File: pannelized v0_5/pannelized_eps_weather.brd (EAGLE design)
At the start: 95.5 x 64 mm, 169 parts, among them IC1 OPA2333DGK, IC100 OPA2333DGK, IC101 OPA347, IC2 OPA2333DGK, Q1 N-HEXFET-2D_SOT232-, Q100 N-HEXFET-2D_SOT232-, Q2 N-HEXFET-2D_SOT232-, Q3 FC-12M, Q4 32.768kHz, Q5 32.768kHz, U1 BMP180, U10 ML8511-UV-SENSORSMD, U11 AS3935, U12 BNO055A, U2 SHT21, U3 ML8511-UV-SENSORSMD, U4 MCP3425, U5 BNO055A, U6 AS3935, U7 SHT21, U8 BMP180, U9 MCP3425

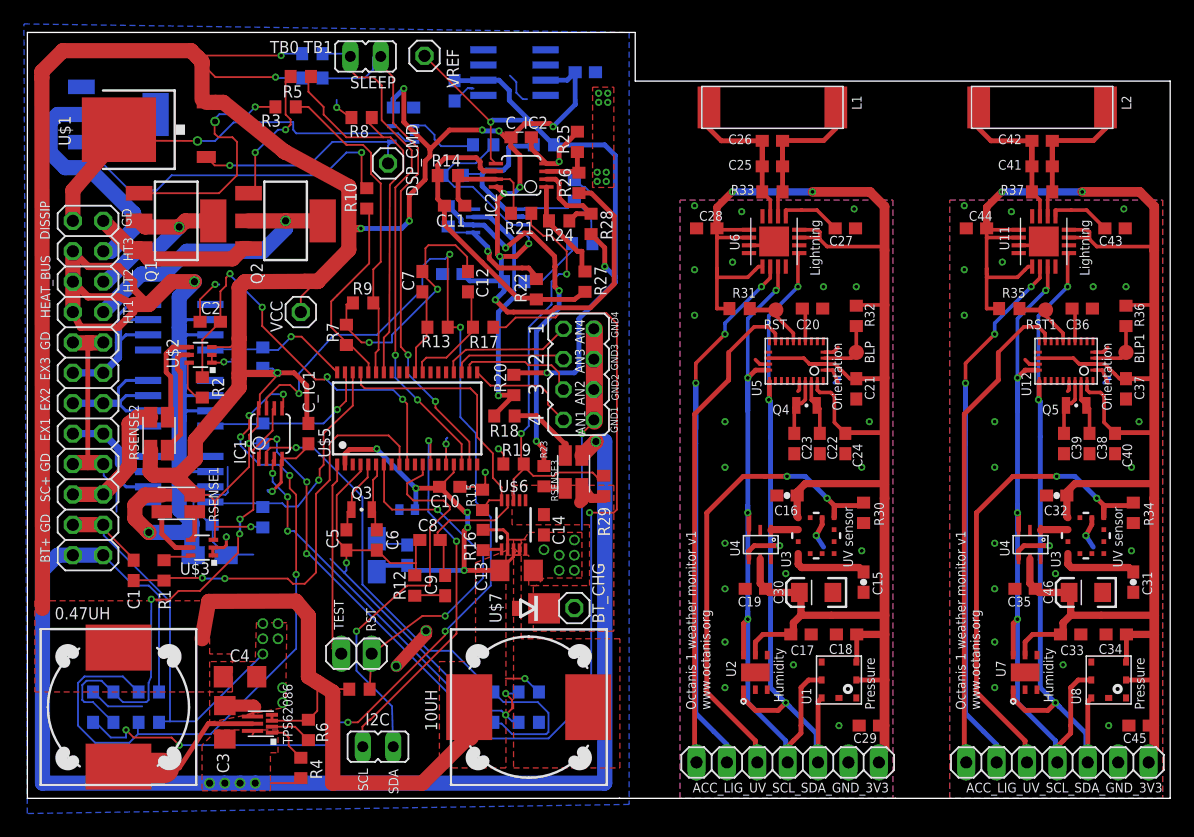
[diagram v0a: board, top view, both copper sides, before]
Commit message: created bom for v0.5
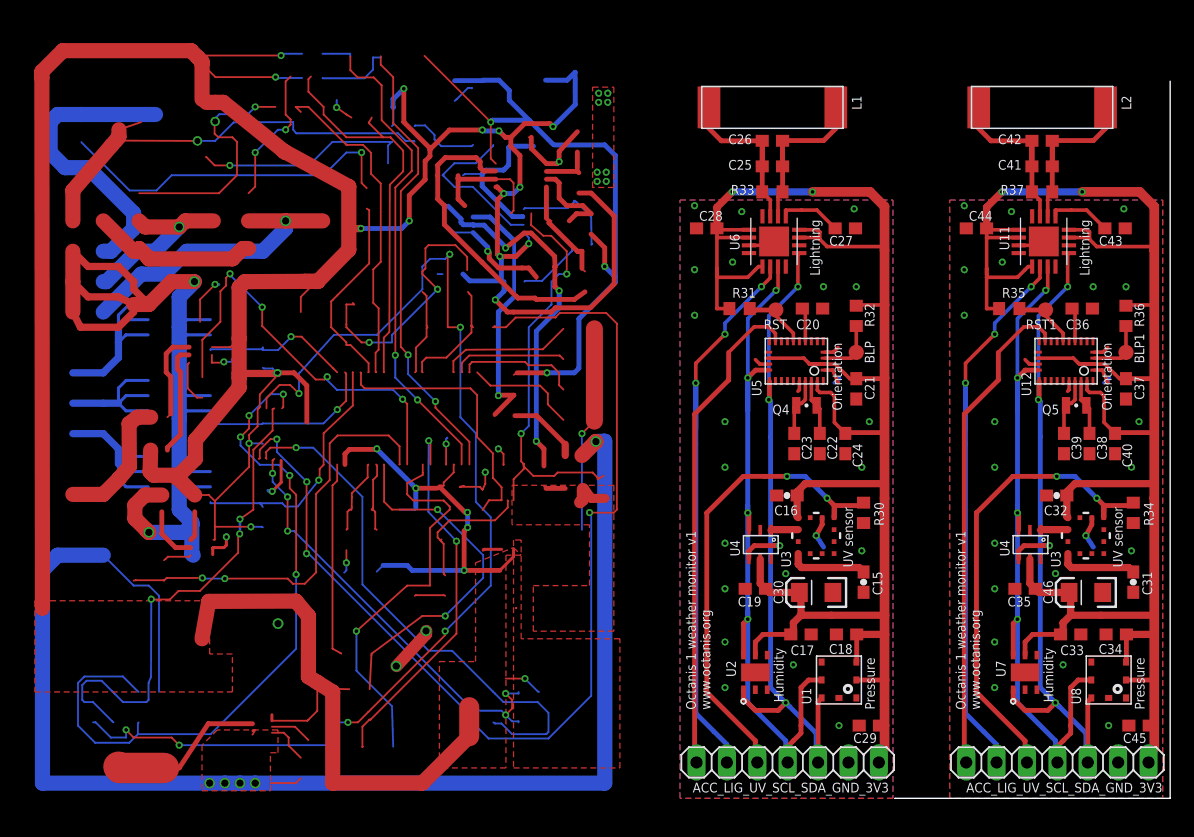
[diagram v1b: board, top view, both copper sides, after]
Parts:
- removed 0.47UH, 10UH: DR127, inductors:DR127
- removed BT_CHG, DSP_CMD, VCC, VREF: (no value), pinhead:1X01
- removed C1, C12, C2, C7: 1.5uF, rcl:C0603
- removed C10, C100, C102, C105, C_IC1, C_IC100, C_IC101, C_IC2: 100nF, rcl:C0603
- removed C101: 2.2nF, rcl:C0603
- removed C103: 10uF, rcl:A/3216-18R
- removed C104: 22uF, rcl:A/3216-18R
- removed C11: 10nF, rcl:C0603
- removed C13: 4.7u, rcl:C1206
- removed C14: 22u, rcl:C0603
- removed C3: 10u, rcl:C1206
- removed C4: 22u, rcl:C1206
- removed C5, C6: 12pF, rcl:C0603
- removed C8: 4.7p, rcl:C0603
- removed C9: 470p, rcl:C0603
- removed FERRITE: 100mH, inductors:0402
- removed I2C, SLEEP: (no value), jumper:JP1
- removed IC1, IC100, IC2: OPA2333DGK, linear:MSOP08
- removed IC101: OPA347, Octanis1_EPS:SC70-5
- removed JP1: (no value), pinhead:2X12
- removed JP2: d SBW clk, pinhead:1X02
- removed JP3: (no value), jumper:JP4Q
- removed Q1, Q100, Q2: N-HEXFET-2D_SOT232-, transistor-power:SOT223
- removed Q3: FC-12M, crystal:FC-12M
- removed R1, R10, R13, R17, R2, R3, R5: 1k, rcl:R0603
- removed R100: 953, rcl:R0603
- removed R101: 86k6, rcl:R0603
- removed R102: 4k02, rcl:R0603
- removed R103, R107, R116, R118, R29: 200k, rcl:R0603
- removed R104, R108, R111, R112, R117, R119, R15, R19: 100k, rcl:R0603
- removed R105: 147k, rcl:R0603
- removed R106: 3k32, rcl:R0603
- removed R109, R21: 560k, rcl:R0603
- removed R11, R18, R23: 10k, rcl:R0603
- removed R110, R20: 920k, rcl:R0603
- removed R113, R114, R115, R24, R6, R7, R8, R9: 1M, rcl:R0603
- removed R12: 82k, rcl:R0603
- removed R14, R22, R27: 162k, rcl:R0603
- removed R16: 30.1k, rcl:R0603
- removed R25: 20k, rcl:R0603
- removed R26: 31.60k, rcl:R0603
- removed R28: 23.2k, rcl:R0603
- removed R4: 0Ohm, rcl:R0603
- removed RSENSE1: RSENSE2, Octanis1_EPS:4PADS_RESISTOR
- removed RSENSE2: RSENSE3, Octanis1_EPS:4PADS_RESISTOR
- removed R_SENSE1: RSENSE1, Octanis1_EPS:4PADS_RESISTOR
- removed U$1: MJD44H11T0-252, Octanis1_EPS:TO252
- removed U$100: MAX6190BESA, Octanis1_EPS:SO8
- removed U$101, U$102, U$103: TPS2022D, Octanis1_EPS:SO8
- removed U$2, U$3: INA213, Octanis1_EPS:SC70-6
- removed U$4: TPS62086, Octanis1_EPS:QFN-7
- removed U$5: MSP430G2544, Octanis1_EPS:TSSOP38_MSPGXX44_SERIES
- removed U$6: LTC3402, Octanis1_EPS:MSOP10
- removed U$7: MBRM120LTIG, Octanis1_EPS:DO216AA
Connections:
- removed net A_EXT1: JP3.7, U$5.20
- removed net A_EXT2: JP3.5, U$5.21
- removed net A_EXT3: JP3.3, U$5.22
- removed net A_EXT4: JP3.1, U$5.23
- removed net BT+: C3.2, JP1.1, JP1.2, R116.2, R4.1, RSENSE2.V1, U$4.7
- removed net BT_CHG: BT_CHG.1, C14.2, R29.1, RSENSE2.V2, U$6.7, U$7.C
- removed net CHG_CMD: C11.1, IC2.7, R14.2, R21.2
- removed net DISSIP: IC101.3, JP1.24, U$1.3
- removed net EN_CHG: R15.1, U$5.35, U$6.10
- removed net EN_EXT1: R115.2, U$103.4, U$5.36
- removed net EN_EXT2: R114.2, U$102.4, U$5.37
- removed net EN_EXT3: R113.2, U$101.4, U$5.38
- removed net EN_HEAT1: R5.2, R8.1, U$5.32
- removed net EN_HEAT2: R3.2, R9.1, U$5.33
- removed net EN_HEAT3: R10.2, R7.1, U$5.34
- removed net EXT1+: JP1.10, JP1.9, U$103.6, U$103.7, U$103.8
- removed net EXT2+: JP1.11, JP1.12, U$102.6, U$102.7, U$102.8
- removed net EXT3+: JP1.13, JP1.14, U$101.6, U$101.7, U$101.8
- removed net EXT_PW: C104.+, C105.2, JP1.18, JP1.20, JP1.22, R_SENSE1.I2, U$101.2, U$101.3, U$102.2, U$102.3, U$103.2, U$103.3
- removed net GND: C1.1, C10.1, C100.1, C101.1, C102.2, C103.-, C104.-, C105.1, C12.1, C13.1, C14.1, C2.1, C3.1, C4.1, C5.2, C6.2, C7.1, C8.1, C_IC1.1, C_IC100.1, C_IC101.1, C_IC2.1, IC1.4, IC100.4, IC101.2, IC2.4, JP1.15, JP1.16, JP1.23, JP1.3, JP1.4, JP1.7, JP1.8, JP3.2, JP3.4, JP3.6, JP3.8, Q1.3, Q100.3, Q2.3, R101.2, R104.1, R107.2, R117.1, R118.2, R12.2, R15.2, R16.2, R19.1, R25.2, R7.2, R8.2, R9.2, U$100.4, U$101.1, U$102.1, U$103.1, U$2.1, U$2.2, U$3.1, U$3.2, U$4.5, U$5.15, U$5.4, U$6.2, U$6.5
- removed net HEAT1: JP1.17, Q2.2, Q2.4
- removed net HEAT2: JP1.19, Q1.2, Q1.4
- removed net HEAT3: JP1.21, Q100.2, Q100.4
- removed net I2C_SCL: I2C.1, U$5.13
- removed net I2C_SDA: I2C.2, U$5.12
- removed net I_EXT_PW: C1.2, R1.1, U$5.9
- removed net I_SC: C2.2, R2.1, U$5.10
- removed net N$1: R1.2, U$3.6
- removed net N$10: IC1.7, R119.1, R13.2
- removed net N$11: C11.2, IC2.6, R14.1, R22.2, R27.2
- removed net N$12: IC1.1, R108.1, R17.2
- removed net N$13: IC1.2, R107.1, R108.2
- removed net N$14: IC1.3, R103.1, R104.2
- removed net N$15: IC1.6, R118.1, R119.2
- removed net N$16: IC1.5, R116.1, R117.2
- removed net N$17: IC100.2, R110.1, R23.2
- removed net N$18: R100.1, R105.2
- removed net N$19: IC100.5, R100.2, R101.1
- removed net N$2: R2.2, U$2.6
- removed net N$20: IC100.6, R102.1, R109.2
- removed net N$21: IC100.7, R106.2, R109.1
- removed net N$22: IC101.1, R106.1
- removed net N$23: R19.2, R21.1, R29.2, U$6.8
- removed net N$24: 10UH.2, U$6.4, U$7.A
- removed net N$25: R6.2, U$4.2
- removed net N$26: 0.47UH.1, U$4.6
- removed net N$28: IC100.3, R18.2, R20.1
- removed net N$29: Q2.1, R5.1
- removed net N$3: R16.1, U$6.1
- removed net N$30: R4.2, U$4.1
- removed net N$31: Q1.1, R3.1
- removed net N$32: R_SENSE1.V1, U$3.4
- removed net N$33: R_SENSE1.V2, U$3.5
- removed net N$34: RSENSE1.V1, U$2.4
- removed net N$35: RSENSE1.V2, U$2.5
- removed net N$37: Q100.1, R10.1
- removed net N$38: R23.1, RSENSE2.I2
- removed net N$4: C9.1, R12.1
- removed net N$40: R18.1, RSENSE2.I1
- removed net N$45: DSP_CMD.1, IC101.4, U$1.1
- removed net N$48: C5.1, Q3.2, U$5.5
- removed net N$5: IC100.1, R110.2, R22.1
- removed net N$50: C6.1, Q3.1, U$5.6
- removed net N$6: IC2.3, R25.1, R26.2
- removed net N$7: IC2.2, R24.1, R28.1
- removed net N$8: C8.2, C9.2, U$6.9
- removed net N$9: IC2.1, R24.2, R27.1
- removed net RST/SBWTDIO: JP2.1, R11.2, U$5.7
- removed net SC+: JP1.5, JP1.6, RSENSE1.I1
- removed net TB0: R111.1, SLEEP.2, U$5.17
- removed net TB1: R112.1, SLEEP.1, U$5.18
- removed net TEST/SBWTCK: JP2.2, U$5.1
- removed net VCC: 0.47UH.2, 10UH.1, C10.2, C100.2, C102.1, C103.+, C13.2, C4.2, C_IC1.2, C_IC100.2, C_IC101.2, C_IC2.2, FERRITE.1, FERRITE.2, IC1.8, IC100.8, IC101.6, IC2.8, R103.2, R105.1, R11.1, R111.2, R112.2, R113.1, R114.1, R115.1, R26.1, R6.1, RSENSE1.I2, R_SENSE1.I1, U$1.2, U$100.3, U$2.3, U$3.3, U$4.3, U$4.4, U$5.16, U$5.2, U$6.3, VCC.1
- removed net VREF: C101.2, IC2.5, R102.2, R20.2, R28.2, U$100.6, VREF.1
- removed net V_BT_MS: C7.2, R13.1, U$5.28
- removed net V_BUS_MS: C12.2, R17.1, U$5.27
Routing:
- net GND: track 225.1 -> 91.6 mm, vias 36 -> 24
- removed copper zone on layer 16, net GND
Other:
- board size 95.5 x 64 mm -> 23 x 59.9 mm
- board text removed: "AN1"
- board text removed: "AN2"
- board text removed: "AN3"
- board text removed: "AN4"
- board text removed: "BT+"
- board text removed: "DISSIP"
- board text removed: "EX1"
- board text removed: "EX2"
- board text removed: "EX3"
- board text removed: "GD"
- board text removed: "GND1"
- board text removed: "GND2"
- board text removed: "GND3"
- board text removed: "GND4"
- board text removed: "HEAT_BUS"
- board text removed: "HT1"
- board text removed: "HT2"
- board text removed: "HT3"
- board text removed: "Octanis_EPS v0.4"
- board text removed: "RST"
- board text removed: "SC+"
- board text removed: "SCL"
- board text removed: "SDA"
- board text removed: "TB0 TB1"
- board text removed: "TEST"
